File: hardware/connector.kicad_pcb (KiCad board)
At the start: 4 copper layers, 20 x 22 mm, 2 parts, among them J1 AXK5F20347YG, J2 AXK5F20347YG

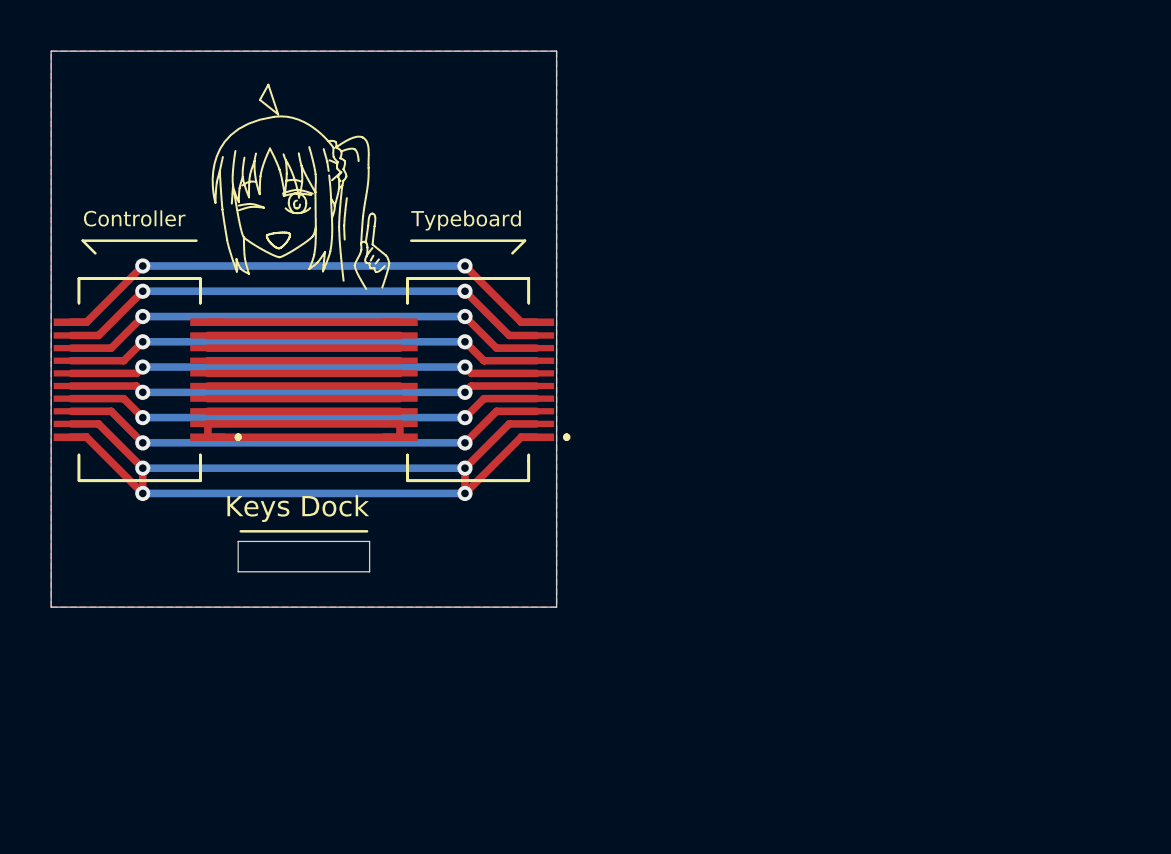
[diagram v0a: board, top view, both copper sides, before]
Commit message: :sparkles: assembly all the part!
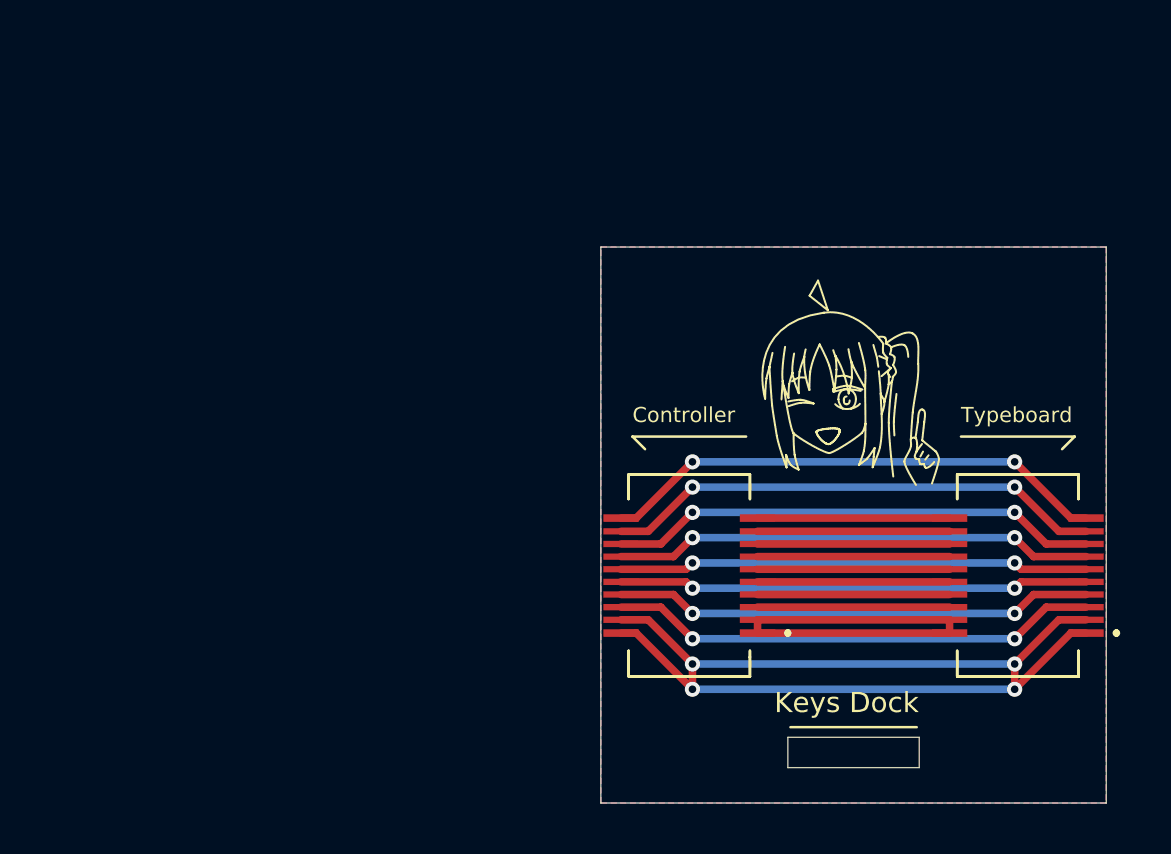
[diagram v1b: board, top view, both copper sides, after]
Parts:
- moved J1 23.1 mm to (140.2, 98.8)
- moved J2 23.1 mm to (153.2, 98.8)
